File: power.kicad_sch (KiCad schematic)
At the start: 23 parts, among them J2 VIN, U6 TPS5430DDA

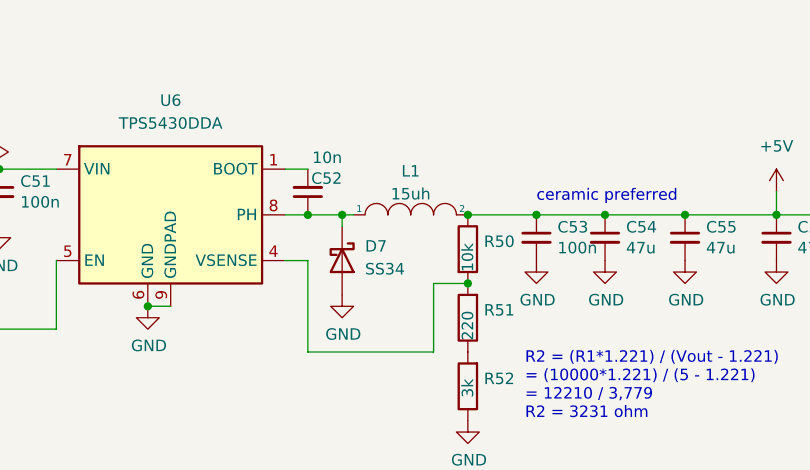
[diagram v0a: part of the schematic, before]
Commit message: Solve all warnings
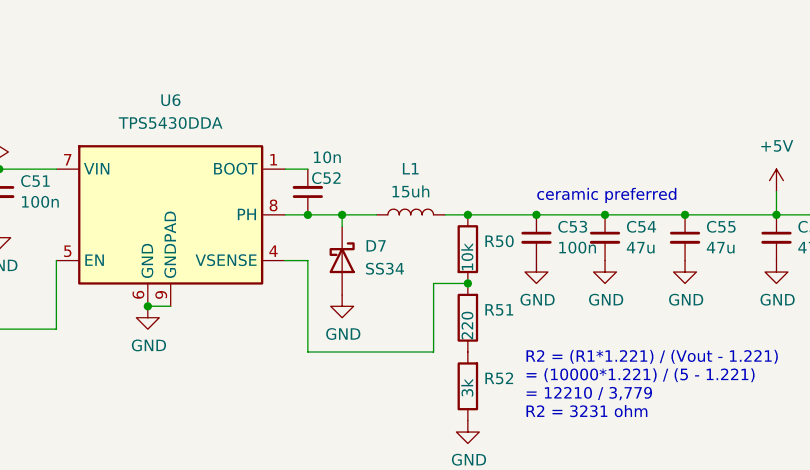
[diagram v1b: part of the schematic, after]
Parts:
- J2: symbol Connector:Conn_01x02_Male -> Connector:Conn_01x02_Pin
- L1: symbol pspice:INDUCTOR -> Device:L
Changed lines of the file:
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@@
+	)
+	(junction
+		(at 149.86 59.69)
+		(diameter 0)
+		(color 0 0 0 0)
 	)
 	(junction
@@
 	)
 	(junction
-		(at 149.86 59.69)
-		(diameter 0)
-		(color 0 0 0 0)
-	)
-	(junction
 		(at 114.3 69.85)
 		(diameter 0)
@@
 	(wire
 		(pts
-			(xy 135.89 59.69) (xy 137.16 59.69)
+			(xy 135.89 59.69) (xy 139.7 59.69)
 		)
 		(stroke
@@
 		(pts
 			(xy 132.08 59.69) (xy 129.54 59.69)
+		)
+		(stroke
+			(width 0)
+			(type default)
+		)
+	)
+	(wire
+		(pts
+			(xy 147.32 59.69) (xy 149.86 59.69)
 		)
 		(stroke
@@
 	)
 	(symbol
-		(lib_id "pspice:INDUCTOR")
-		(at 143.51 59.69 0)
+		(lib_id "Device:L")
+		(at 143.51 59.69 90)
 		(unit 1)
 		(exclude_from_sim no)
@@
 		(fields_autoplaced yes)
 		(property "Reference" "L1"
-			(at 143.51 54.8472 0)
+			(at 143.51 54.61 90)
 			(effects
 				(font
@@
 		)
 		(property "Value" "15uh"
-			(at 143.51 57.3841 0)
+			(at 143.51 57.15 90)
 			(effects
 				(font
@@
 			)
 		)
-		(property "Description" ""
+		(property "Description" "Inductor"
 			(at 143.51 59.69 0)
 			(effects
@@
 	)
 	(symbol
-		(lib_id "Connector:Conn_01x02_Male")
+		(lib_id "Connector:Conn_01x02_Pin")
 		(at 49.53 54.61 0)
 		(unit 1)
@@
 			)
 		)
-		(property "Description" ""
+		(property "Description" "Generic connector, single row, 01x02, script generated"
 			(at 49.53 54.61 0)
 			(effects
